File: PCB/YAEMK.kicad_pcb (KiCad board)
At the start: 2 copper layers, 162.8 x 130.8 mm, 176 parts, among them J1 DBG, P1 PC, P2 Link, P3 SSD1107, Q2 Q_PNP_BCE, SW1 ALPS EC11, U1 USBLC6-2SC6, U2 USBLC6-2SC6, U3 STM32F103CBTx, U4 24LC64, U5 TLV62568DBV

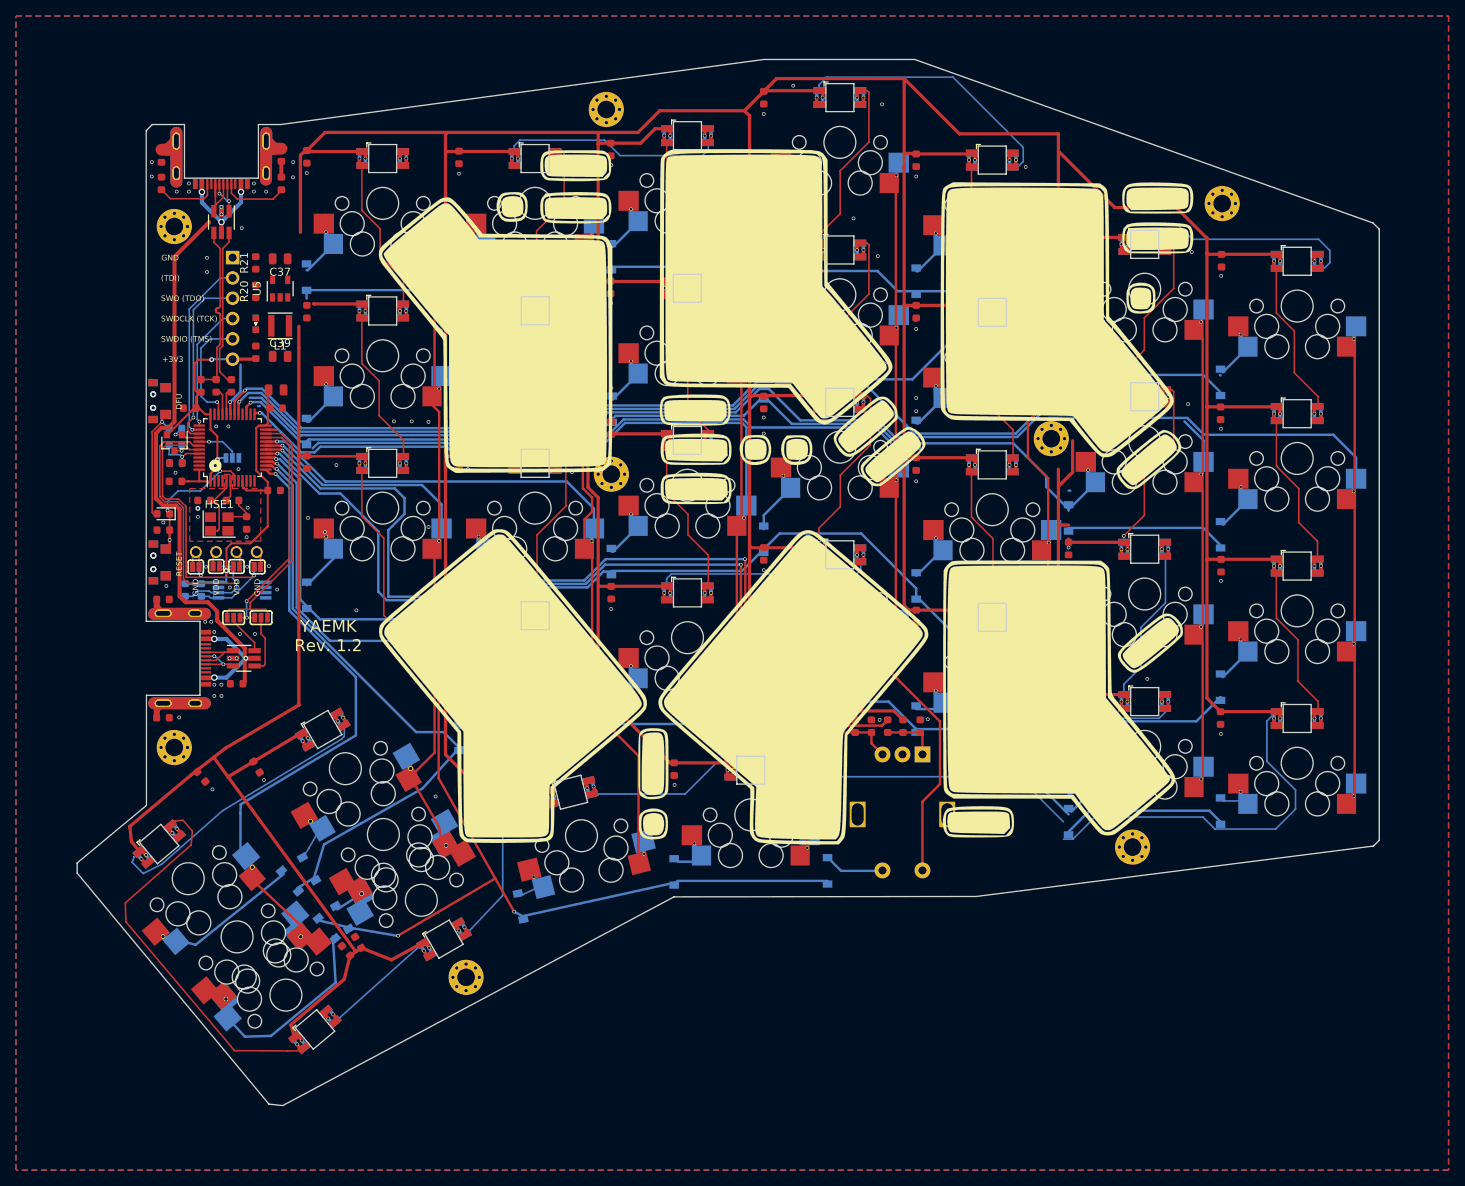
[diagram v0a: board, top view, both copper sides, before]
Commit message: One step further
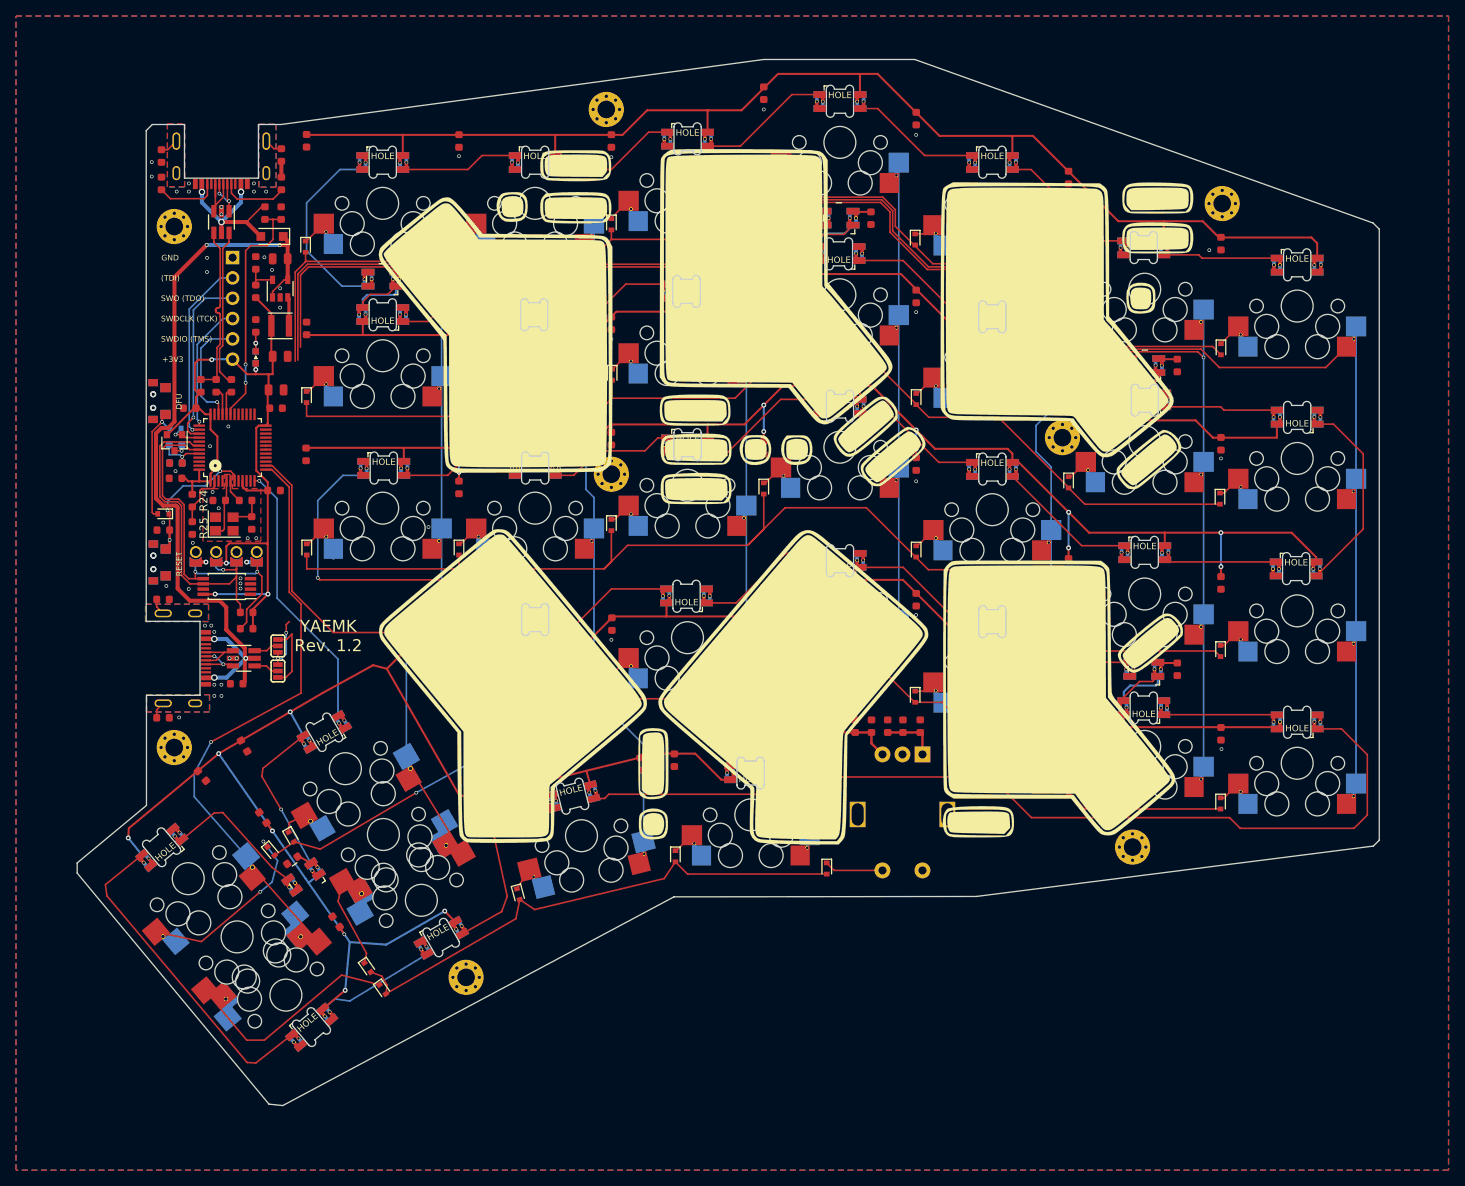
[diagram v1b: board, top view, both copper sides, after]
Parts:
- removed the C21 at (120.8, 121.1)
- removed the C47 at (93.1, 81.3)
- removed the D11 at (116.2, 94.7)
- removed the D4 at (101.6, 134.6)
- removed JP10, JP3, JP4, JP5, JP6, JP7, JP8, JP9: SolderJumper_2_Open, prettylib:SOLDER_JUMPER_2
- removed JP11: HANDNESS, prettylib:SOLDER_JUMPER_3
- added C13: 100n, prettylib:SMD-0603, F.Cu at (153.2, 111.3)
- added C39: 100n, prettylib:SMD-0603, F.Cu at (93.1, 81.3)
- added C48: 100n, prettylib:SMD-0603, F.Cu at (139.1, 115.4)
- added C49: 100n, prettylib:SMD-0603, F.Cu at (206.0, 103.6)
- added C50: 100n, prettylib:SMD-0603, F.Cu at (206.0, 65.7)
- added C51: 100n, prettylib:SMD-0603, F.Cu at (167.7, 47.2)
- added C52: 100n, prettylib:SMD-0603, F.Cu at (110.6, 54.9)
- added C53: 100n, prettylib:SMD-0603, F.Cu at (95.4, 127.5)
- added D10: DIODE, Diode_SMD:D_SOD-523, F.Cu at (116.2, 88.6)
- added D35: SW, prettylib:SK6812_mini_e_flippable, F.Cu at (99.3, 111.4)
- added D36: SW, prettylib:SK6812_mini_flipable, F.Cu at (96.8, 129.6)
- added D37: SW, prettylib:SK6812_mini_e_flippable, B.Cu at (79.1, 126.0)
- added D38: SW, prettylib:SK6812_mini_e_flippable, F.Cu at (97.9, 148.5)
- added D39: SW, prettylib:SK6812_mini_e_flippable, F.Cu at (114.0, 137.3)
- added D40: SW, prettylib:SK6812_mini_e_flippable, F.Cu at (130.4, 119.6)
- added D41: SW, prettylib:SK6812_mini_flipable, F.Cu at (157.2, 111.3)
- added D42: SW, prettylib:SK6812_mini_e_flippable, F.Cu at (152.7, 116.5)
- added D43: SW, prettylib:SK6812_mini_flipable, F.Cu at (201.8, 103.6)
- added D44: SW, prettylib:SK6812_mini_e_flippable, F.Cu at (201.8, 108.3)
- added D45: SW, prettylib:SK6812_mini_e_flippable, F.Cu at (182.9, 97.5)
- added D46: SW, prettylib:SK6812_mini_e_flippable, F.Cu at (221.0, 110.1)
- added D47: SW, prettylib:SK6812_mini_e_flippable, F.Cu at (163.8, 89.9)
- added D48: SW, prettylib:SK6812_mini_e_flippable, F.Cu at (144.7, 94.4)
- added D49: SW, prettylib:SK6812_mini_e_flippable, F.Cu at (125.7, 97.3)
- added D50: SW, prettylib:SK6812_mini_e_flippable, F.Cu at (106.8, 78.6)
- added D51: SW, prettylib:SK6812_mini_e_flippable, F.Cu at (125.7, 78.6)
- added D52: SW, prettylib:SK6812_mini_e_flippable, F.Cu at (144.8, 75.7)
- added D53: SW, prettylib:SK6812_mini_e_flippable, F.Cu at (163.8, 70.9)
- added D54: SW, prettylib:SK6812_mini_e_flippable, F.Cu at (182.9, 78.7)
- added D55: SW, prettylib:SK6812_mini_e_flippable, F.Cu at (201.9, 89.2)
- added D56: SW, prettylib:SK6812_mini_e_flippable, F.Cu at (220.9, 91.2)
- added D57: SW, prettylib:SK6812_mini_e_flippable, F.Cu at (221.0, 72.0)
- added D58: SW, prettylib:SK6812_mini_e_flippable, F.Cu at (201.9, 69.8)
- added D59: SW, prettylib:SK6812_mini_flipable, F.Cu at (201.9, 65.7)
- added D60: SW, prettylib:SK6812_mini_e_flippable, F.Cu at (182.9, 59.4)
- added D61: SW, prettylib:SK6812_mini_e_flippable, F.Cu at (163.7, 51.6)
- added D62: SW, prettylib:SK6812_mini_flipable, F.Cu at (163.7, 47.2)
- added D63: SW, prettylib:SK6812_mini_e_flippable, F.Cu at (144.7, 56.3)
- added D64: SW, prettylib:SK6812_mini_e_flippable, F.Cu at (125.6, 59.2)
- added D65: SW, prettylib:SK6812_mini_flipable, F.Cu at (106.6, 54.9)
- added D66: SW, prettylib:SK6812_mini_e_flippable, F.Cu at (106.7, 59.2)
- added D67: SW, prettylib:SK6812_mini_e_flippable, F.Cu at (106.7, 40.4)
- added D7: DIODE, Diode_SMD:D_SOD-523, F.Cu at (104.8, 140.9)
- added D71: SW, prettylib:SK6812_mini_e_flippable, F.Cu at (125.7, 40.4)
- added D72: SW, prettylib:SK6812_mini_e_flippable, F.Cu at (144.8, 37.5)
- added D73: SW, prettylib:SK6812_mini_e_flippable, F.Cu at (163.8, 32.8)
- added D74: SW, prettylib:SK6812_mini_e_flippable, F.Cu at (182.9, 40.4)
- added D75: SW, prettylib:SK6812_mini_e_flippable, F.Cu at (201.8, 51.1)
- added D76: SW, prettylib:SK6812_mini_e_flippable, F.Cu at (221.0, 53.2)
- added D77: D_Schottky, Diode_SMD:D_SOD-123F, F.Cu at (92.8, 49.5)
- added R22: 1k5, prettylib:SMD-0603, F.Cu at (91.9, 46.6)
- added R23: 1k5, prettylib:SMD-0603, F.Cu at (94.0, 46.6)
- added R24: 1k5, prettylib:SMD-0603, F.Cu at (82.9, 82.5)
- added R25: 1k5, prettylib:SMD-0603, F.Cu at (82.9, 86.0)
- D1, D2: footprint Diode_SMD:D_SOD-123 -> Diode_SMD:D_SOD-523; moved to F.Cu
- D11: renamed from D12; footprint Diode_SMD:D_SOD-123 -> Diode_SMD:D_SOD-523; moved to F.Cu
- D12: renamed from D13; footprint Diode_SMD:D_SOD-123 -> Diode_SMD:D_SOD-523; moved to F.Cu
- D13: renamed from D14; footprint Diode_SMD:D_SOD-123 -> Diode_SMD:D_SOD-523; moved to F.Cu
- D14: renamed from D15; footprint Diode_SMD:D_SOD-123 -> Diode_SMD:D_SOD-523; moved to F.Cu
- D15: renamed from D16; footprint Diode_SMD:D_SOD-123 -> Diode_SMD:D_SOD-523; moved to F.Cu
- D16: renamed from D17; footprint Diode_SMD:D_SOD-123 -> Diode_SMD:D_SOD-523; moved to F.Cu
- D17: renamed from D18; footprint Diode_SMD:D_SOD-123 -> Diode_SMD:D_SOD-523; moved to F.Cu
- D18: renamed from D19; footprint Diode_SMD:D_SOD-123 -> Diode_SMD:D_SOD-523; moved to F.Cu
- D19: renamed from D20; footprint Diode_SMD:D_SOD-123 -> Diode_SMD:D_SOD-523; moved to F.Cu
- D20: renamed from D21; footprint Diode_SMD:D_SOD-123 -> Diode_SMD:D_SOD-523; moved to F.Cu
- D21: renamed from D22; footprint Diode_SMD:D_SOD-123 -> Diode_SMD:D_SOD-523; moved to F.Cu
- D22: renamed from D23; footprint Diode_SMD:D_SOD-123 -> Diode_SMD:D_SOD-523; moved to F.Cu
- D23: renamed from D24; footprint Diode_SMD:D_SOD-123 -> Diode_SMD:D_SOD-523; moved to F.Cu
- D24: renamed from D25; footprint Diode_SMD:D_SOD-123 -> Diode_SMD:D_SOD-523; moved to F.Cu
- D25: renamed from D26; footprint Diode_SMD:D_SOD-123 -> Diode_SMD:D_SOD-523; moved to F.Cu
- D26: renamed from D27; footprint Diode_SMD:D_SOD-123 -> Diode_SMD:D_SOD-523; moved to F.Cu
- D27: renamed from D29; footprint Diode_SMD:D_SOD-123 -> Diode_SMD:D_SOD-523; moved to F.Cu
- D28: renamed from D30; footprint Diode_SMD:D_SOD-123 -> Diode_SMD:D_SOD-523; moved to F.Cu
- D29: renamed from D31; footprint Diode_SMD:D_SOD-123 -> Diode_SMD:D_SOD-523; moved to F.Cu
- D3: renamed from D5; footprint Diode_SMD:D_SOD-123 -> Diode_SMD:D_SOD-523; moved to F.Cu
- D30: renamed from D32; footprint Diode_SMD:D_SOD-123 -> Diode_SMD:D_SOD-523; moved to F.Cu
- D31: renamed from D34; footprint Diode_SMD:D_SOD-123 -> Diode_SMD:D_SOD-523; moved to F.Cu
- D32: renamed from D35; footprint Diode_SMD:D_SOD-123 -> Diode_SMD:D_SOD-523; moved to F.Cu
- D33: renamed from D36; footprint Diode_SMD:D_SOD-123 -> Diode_SMD:D_SOD-523; moved to F.Cu
- D34: renamed from D37; footprint Diode_SMD:D_SOD-123 -> Diode_SMD:D_SOD-523; moved to F.Cu
- D4: renamed from D6; footprint Diode_SMD:D_SOD-123 -> Diode_SMD:D_SOD-523; moved to F.Cu
- D5: renamed from D7; footprint Diode_SMD:D_SOD-123 -> Diode_SMD:D_SOD-523; moved to F.Cu
- D6: renamed from D3; footprint Diode_SMD:D_SOD-123 -> Diode_SMD:D_SOD-523; moved to F.Cu
- D68: renamed from D38; footprint Diode_SMD:D_0603_1608Metric -> Diode_SMD:D_SOD-523
- D69: renamed from D39; footprint Diode_SMD:D_0603_1608Metric -> Diode_SMD:D_SOD-523
- D8: renamed from D9; footprint Diode_SMD:D_SOD-123 -> Diode_SMD:D_SOD-523; moved to F.Cu
- D9: renamed from D10; footprint Diode_SMD:D_SOD-123 -> Diode_SMD:D_SOD-523; moved to F.Cu
- R7: renamed from R9; moved to F.Cu
- R8: renamed from R14; moved to F.Cu
- S1, S5: footprint prettylib:MX_KAILH_SOCKET_WS2812_2U_2X1U -> prettylib:MX_KAILH_SOCKET_2U_2X1U
- S10: renamed from S13; footprint prettylib:MX_KAILH_SOCKET_SK9822_1U -> prettylib:MX_KAILH_SOCKET_1U
- S11: renamed from S14; footprint prettylib:MX_KAILH_SOCKET_SK9822_1U -> prettylib:MX_KAILH_SOCKET_1U
- S12: renamed from S15; footprint prettylib:MX_KAILH_SOCKET_SK9822_1U -> prettylib:MX_KAILH_SOCKET_1U
- S13: renamed from S16; footprint prettylib:MX_KAILH_SOCKET_SK9822_1U -> prettylib:MX_KAILH_SOCKET_1U
- S14: renamed from S17; footprint prettylib:MX_KAILH_SOCKET_SK9822_1U -> prettylib:MX_KAILH_SOCKET_1U
- S15: renamed from S18; footprint prettylib:MX_KAILH_SOCKET_SK9822_1U -> prettylib:MX_KAILH_SOCKET_1U
- S16: renamed from S19; footprint prettylib:MX_KAILH_SOCKET_SK9822_1U -> prettylib:MX_KAILH_SOCKET_1U
- S17: renamed from S20; footprint prettylib:MX_KAILH_SOCKET_SK9822_1U -> prettylib:MX_KAILH_SOCKET_1U
- S18: renamed from S21; footprint prettylib:MX_KAILH_SOCKET_SK9822_1U -> prettylib:MX_KAILH_SOCKET_1U
- S19: renamed from S22; footprint prettylib:MX_KAILH_SOCKET_SK9822_1U -> prettylib:MX_KAILH_SOCKET_1U
- S2, S3, S4: footprint prettylib:MX_KAILH_SOCKET_SK9822_1U -> prettylib:MX_KAILH_SOCKET_1U
- S20: renamed from S24; footprint prettylib:MX_KAILH_SOCKET_SK9822_1U -> prettylib:MX_KAILH_SOCKET_1U
- S21: renamed from S25; footprint prettylib:MX_KAILH_SOCKET_SK9822_1U -> prettylib:MX_KAILH_SOCKET_1U
- S22: renamed from S26; footprint prettylib:MX_KAILH_SOCKET_SK9822_1U -> prettylib:MX_KAILH_SOCKET_1U
- S23: renamed from S27; footprint prettylib:MX_KAILH_SOCKET_SK9822_1U -> prettylib:MX_KAILH_SOCKET_1U
- S24: renamed from S28; footprint prettylib:MX_KAILH_SOCKET_SK9822_1U -> prettylib:MX_KAILH_SOCKET_1U
- S25: renamed from S29; footprint prettylib:MX_KAILH_SOCKET_SK9822_1U -> prettylib:MX_KAILH_SOCKET_1U
- S26: renamed from S30; footprint prettylib:MX_KAILH_SOCKET_SK9822_1U -> prettylib:MX_KAILH_SOCKET_1U
- S27: renamed from S31; footprint prettylib:MX_KAILH_SOCKET_SK9822_1U -> prettylib:MX_KAILH_SOCKET_1U
- S28: renamed from S32; footprint prettylib:MX_KAILH_SOCKET_SK9822_1U -> prettylib:MX_KAILH_SOCKET_1U
- S29: renamed from S33; footprint prettylib:MX_KAILH_SOCKET_SK9822_1U -> prettylib:MX_KAILH_SOCKET_1U
- S30: renamed from S34; footprint prettylib:MX_KAILH_SOCKET_SK9822_1U -> prettylib:MX_KAILH_SOCKET_1U
- S31: renamed from S35; footprint prettylib:MX_KAILH_SOCKET_SK9822_1U -> prettylib:MX_KAILH_SOCKET_1U
- S6: renamed from S9; footprint prettylib:MX_KAILH_SOCKET_SK9822_1U -> prettylib:MX_KAILH_SOCKET_1U
- S7: renamed from S10; footprint prettylib:MX_KAILH_SOCKET_SK9822_1U -> prettylib:MX_KAILH_SOCKET_1U
- S8: renamed from S11; footprint prettylib:MX_KAILH_SOCKET_SK9822_1U -> prettylib:MX_KAILH_SOCKET_1U
- S9: renamed from S12; footprint prettylib:MX_KAILH_SOCKET_SK9822_1U -> prettylib:MX_KAILH_SOCKET_1U
- U1: renamed from U4; moved to F.Cu
- moved C27 19.6 mm to (91.7, 122.2), turned to 125 degrees
- moved D2 10.3 mm to (106.7, 143.6), turned to 305 degrees
- moved MH5 9.91 mm to (164.0, 105.5)
- moved C16 8.25 mm to (192.4, 42.2), turned to 270 degrees
- moved R8 8.18 mm to (89.7, 96.5), turned to 180 degrees
- moved R7 7.43 mm to (89.7, 98.6), turned to 180 degrees
- moved JP2 6.99 mm to (93.6, 103.8), turned to 90 degrees
- moved JP1 6.57 mm to (93.6, 100.7), turned to 270 degrees
- moved D20 6.35 mm to (154.3, 81.0)
- moved D18 6.22 mm to (154.4, 43.2)
- moved D19 6.22 mm to (154.3, 62.0)
- moved D5 5.74 mm to (97.2, 88.6)
- moved C34 5.66 mm to (154.3, 75.9), turned to 270 degrees
- moved D23 5.21 mm to (173.2, 49.9)
- moved C6 5.21 mm to (173.4, 34.8), turned to 270 degrees
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- renumbered C18 to C11, C14 to C12, C12 to C14, C20 to C15, C17 to C16, C23 to C17, C19 to C18, C13 to C19, C22 to C20, C24 to C21, C16 to C22, C25 to C23, C15 to C24, C26 to C25, C30 to C26, C4 to C3, C33 to C30, C35 to C31, C31 to C32, C32 to C33, C36 to C35, C42 to C36, C43 to C37, C45 to C38, C5 to C4, C3 to C40, C49 to C41, C38 to C42, C37 to C43, C39 to C44, C60 to C45, C57 to C46, C59 to C47, C6 to C5, C7 to C6, C8 to C7, C9 to C8, C11 to C9, D77 to D70, MH2 to MH1, MH4 to MH2, MH6 to MH3, MH8 to MH4, MH9 to MH5, MH1 to MH6, MH3 to MH7, MH5 to MH8, MH7 to MH9, Q2 to Q1, R18 to R1, R4 to R10, R8 to R11, R3 to R12, R2 to R13, R10 to R14, R20 to R15, R21 to R16, R6 to R17, R15 to R18, R16 to R19, R12 to R2, R7 to R20, R13 to R21, R17 to R3, R19 to R4, R1 to R5, R11 to R6, R5 to R9, S7 to S32, S6 to S33, U5 to U2, U1 to U3, U2 to U4, U3 to U5
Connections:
- C10 pad 1: VSS -> VDD
- C10 pad 2: VDD -> VSS
- C11 pad 1: VSS -> VDD
- C11 pad 2: VDD -> VSS
- C12 pad 1: VSS -> VDD
- C12 pad 2: VDD -> VSS
- C14 pad 1: VSS -> VDD
- C14 pad 2: VDD -> VSS
- C15 pad 1: VSS -> VDD
- C15 pad 2: VDD -> VSS
- C16 pad 1: VSS -> VDD
- C16 pad 2: VDD -> VSS
- C17 pad 1: VSS -> VDD
- C17 pad 2: VDD -> VSS
- C18 pad 1: VSS -> VDD
- C18 pad 2: VDD -> VSS
- C19 pad 1: VSS -> VDD
- C19 pad 2: VDD -> VSS
- C20 pad 1: VSS -> VDD
- C20 pad 2: VDD -> VSS
- C21 pad 1: VSS -> VDD
- C21 pad 2: VDD -> VSS
- C22 pad 1: VSS -> VDD
- C22 pad 2: VDD -> VSS
- C23 pad 1: VSS -> VDD
- C23 pad 2: VDD -> VSS
- C24 pad 1: VSS -> VDD
- C24 pad 2: VDD -> VSS
- C25 pad 1: VSS -> VDD
- C25 pad 2: VDD -> VSS
- C26 pad 1: VSS -> VDD
- C26 pad 2: VDD -> VSS
- C27 pad 1: VSS -> VDD
- C27 pad 2: VDD -> VSS
- C28 pad 1: VSS -> VDD
- C28 pad 2: VDD -> VSS
- C29 pad 1: VSS -> VDD
- C29 pad 2: VDD -> VSS
- C3 pad 1: VSS -> VDD
- C3 pad 2: VDD -> VSS
- C30 pad 1: VSS -> VDD
- C30 pad 2: VDD -> VSS
- C31 pad 1: VSS -> VDD
- C31 pad 2: VDD -> VSS
- C32 pad 1: VSS -> VDD
- C32 pad 2: VDD -> VSS
- C33 pad 1: VSS -> VDD
- C33 pad 2: VDD -> VSS
- C34 pad 1: VSS -> VDD
- C34 pad 2: VDD -> VSS
- C35 pad 1: VSS -> VDD
- C35 pad 2: VDD -> VSS
- C4 pad 1: VSS -> VDD
- C4 pad 2: VDD -> VSS
- C43 pad 1: USB_VBUS -> USB_VBUS_IN
- C45 pad 2: USB_VBUS -> USB_VBUS_IN
- C5 pad 1: VSS -> VDD
- C5 pad 2: VDD -> VSS
- C6 pad 1: VSS -> VDD
- C6 pad 2: VDD -> VSS
- C7 pad 1: VSS -> VDD
- C7 pad 2: VDD -> VSS
- C8 pad 1: VSS -> VDD
- C8 pad 2: VDD -> VSS
- C9 pad 1: VSS -> VDD
- C9 pad 2: VDD -> VSS
- P1 pad A8: (no net) -> Net-(P1-PadA8)
- P1 pad B8: (no net) -> Net-(P1-PadB8)
- P2 pad A4: USB_VBUS -> USB_VBUS_IN
- P2 pad A5: (no net) -> Net-(P2-PadA5)
- P2 pad A8: (no net) -> Net-(P2-PadA8)
- P2 pad A9: USB_VBUS -> USB_VBUS_IN
- P2 pad B4: USB_VBUS -> USB_VBUS_IN
- P2 pad B5: (no net) -> Net-(P2-PadB5)
- P2 pad B8: (no net) -> Net-(P2-PadB8)
- P2 pad B9: USB_VBUS -> USB_VBUS_IN
- P3 pad 1: Net-(JP10-Pad2) -> I2C1_SDA
- P3 pad 2: Net-(JP4-Pad2) -> I2C1_SCL
- P3 pad 3: Net-(JP5-Pad2) -> VDD
- P3 pad 4: Net-(JP6-Pad2) -> VSS
- U2 pad 1: USB_VBUS -> USB_VBUS_IN
- U2 pad 4: USB_VBUS -> USB_VBUS_IN
- U4 pad 5: USB_VBUS -> USB_VBUS_IN
- U5 pad 10: (no net) -> Net-(U5-Pad10)
- U5 pad 11: (no net) -> Net-(U5-Pad11)
- U5 pad 12: (no net) -> TIM2_CH3
- U5 pad 14: Row4 -> Col2
- U5 pad 19: Col2 -> Net-(U5-Pad19)
- U5 pad 2: (no net) -> HANDNESS
- U5 pad 26: (no net) -> Net-(U5-Pad26)
- U5 pad 28: (no net) -> Net-(U5-Pad28)
- U5 pad 3: (no net) -> Net-(U5-Pad3)
- U5 pad 31: Row1 -> SPLIT_DETECT
- U5 pad 4: (no net) -> Net-(U5-Pad4)
- U5 pad 41: HANDNESS -> Net-(U5-Pad41)
- U5 pad 45: (no net) -> Net-(U5-Pad45)
- U5 pad 46: (no net) -> Net-(U5-Pad46)
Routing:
- net Col6: track 175.0 -> 62.8 mm, vias 1 -> 0
- net Col5: track 170.8 -> 64.4 mm
- net Rot_B: track 105.2 -> 0.00 mm, vias 2 -> 0
- net Rot_A: track 104.9 -> 0.01 mm, vias 2 -> 0
- net VDD: track 1028.0 -> 923.4 mm, vias 3 -> 22
- net USB_VBUS_IN: track 0.00 -> 97.7 mm, vias 0 -> 5
- net Net-(D41-Pad1): track 0.00 -> 91.6 mm
- net Net-(S18-Pad1): track 84.9 -> 0.00 mm
- net Row5: track 140.2 -> 66.1 mm, vias 4 -> 0
- net Col4: track 162.1 -> 88.0 mm, vias 1 -> 0
- net USB_VBUS: track 94.3 -> 22.0 mm, vias 6 -> 3
- net Net-(S1-Pad1): track 48.6 -> 0.00 mm
- net Net-(D49-Pad2): track 0.00 -> 44.5 mm, vias 0 -> 1
- net Col3: track 129.6 -> 85.5 mm, vias 1 -> 0
- net Net-(S12-Pad1): track 42.9 -> 0.00 mm, vias 1 -> 0
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- added copper zone on B.Cu, net Net-(P1-PadS1)
- added copper zone on F.Cu, net Net-(P1-PadS1)
- added copper zone on B.Cu, net Net-(P2-PadS1)
- added copper zone on F.Cu, net Net-(P2-PadS1)
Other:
- net class MATRIX: trace_width 0.3048 -> 0.2032
- board text removed: "SCL"
- board text removed: "SDA"
- board text removed: "VDD"
